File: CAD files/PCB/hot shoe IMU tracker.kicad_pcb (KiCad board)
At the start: 2 copper layers, 75 x 35 mm, 25 parts, among them J1 USB_B_Micro, J2 Micro_SD_Card, J3 OLED, J4 BNO085, Q1 2N7002, SW1 Power, SW2 Start, SW3 Stop, U1 ESP32-C3_SUPERMINI_TH, U2 TP4056-42-ESOP8

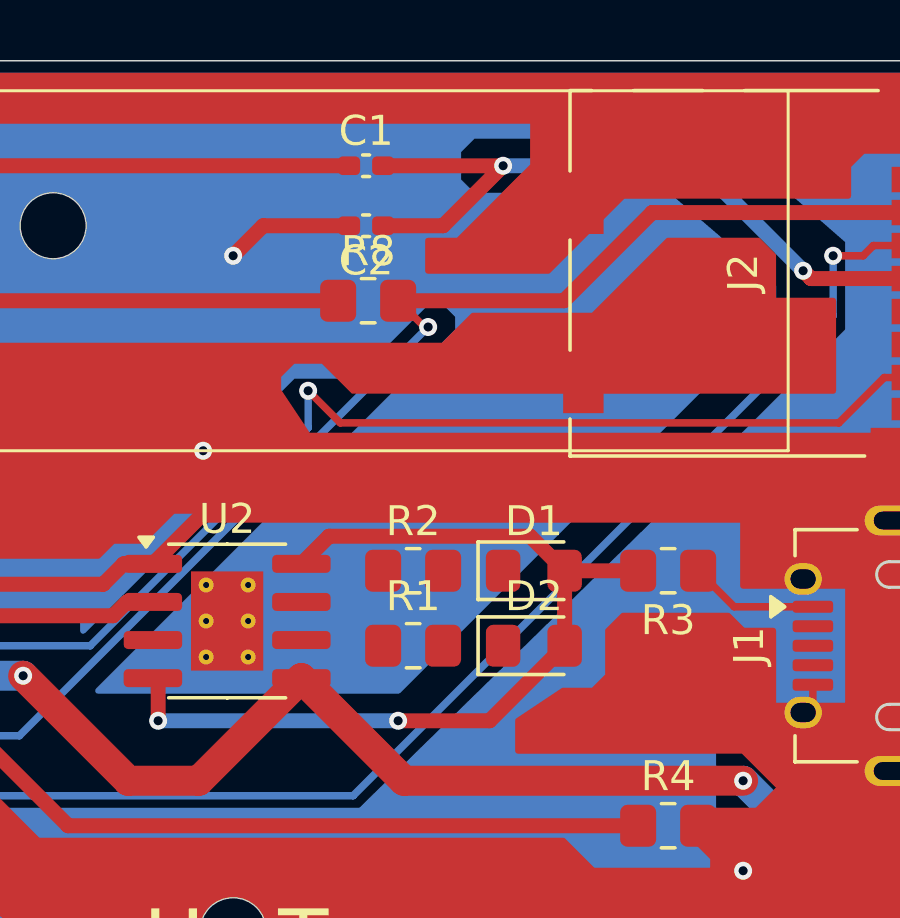
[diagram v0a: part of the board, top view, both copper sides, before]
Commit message: Add files via upload
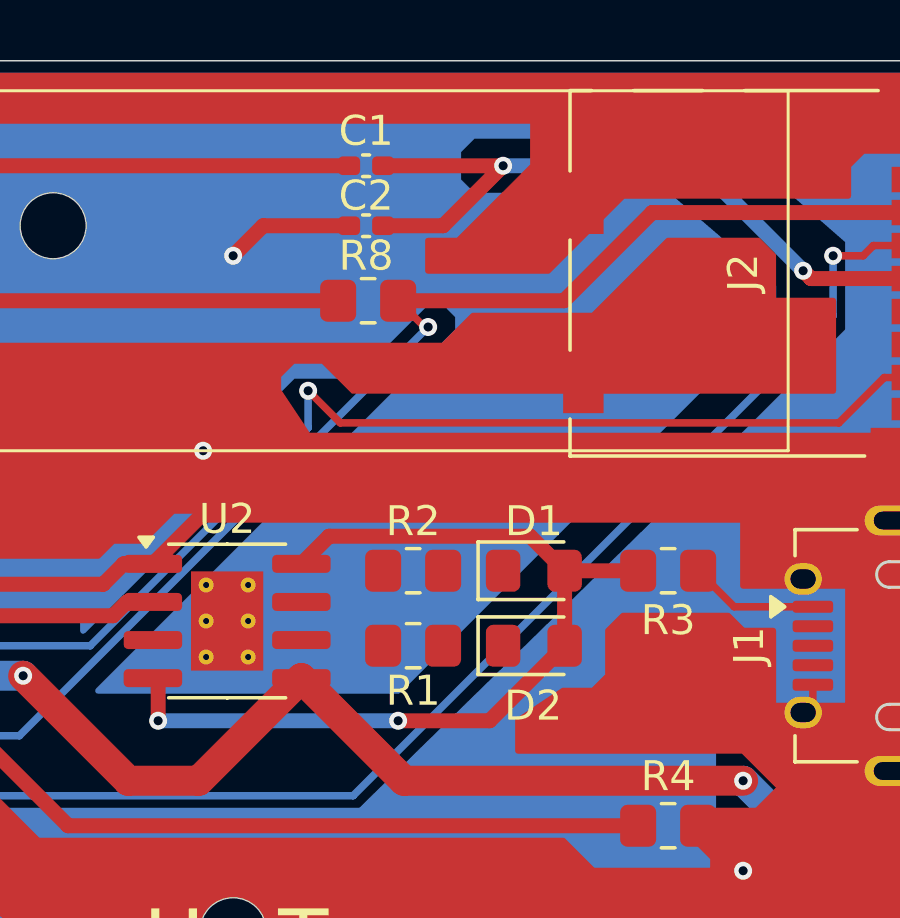
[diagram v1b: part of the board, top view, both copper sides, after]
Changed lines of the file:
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@@
 			(outputformat 1)
 			(mirror no)
-			(drillshape 1)
+			(drillshape 0)
 			(scaleselection 1)
-			(outputdirectory "")
+			(outputdirectory "../")
 		)
 	)
@@
 		(tags "resistor handsolder")
 		(property "Reference" "R8"
-			(at 0 -1.65 0)
+			(at -0.0675 -1.5 0)
 			(layer "F.SilkS")
 			(effects
@@
 		(tags "resistor handsolder")
 		(property "Reference" "R1"
-			(at 0 -1.65 0)
+			(at 0 1.5 0)
 			(layer "F.SilkS")
 			(effects
@@
 		(tags "capacitor handsolder")
 		(property "Reference" "C2"
-			(at 0 -1.16 0)
+			(at 0 1 0)
 			(layer "F.SilkS")
 			(effects
@@
 		(tags "LED handsolder")
 		(property "Reference" "D2"
-			(at 0 -1.65 0)
+			(at -0.025 2 0)
 			(layer "F.SilkS")
 			(effects
